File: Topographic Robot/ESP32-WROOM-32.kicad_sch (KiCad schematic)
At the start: 3 parts, among them U5 ESP32-WROOM-32

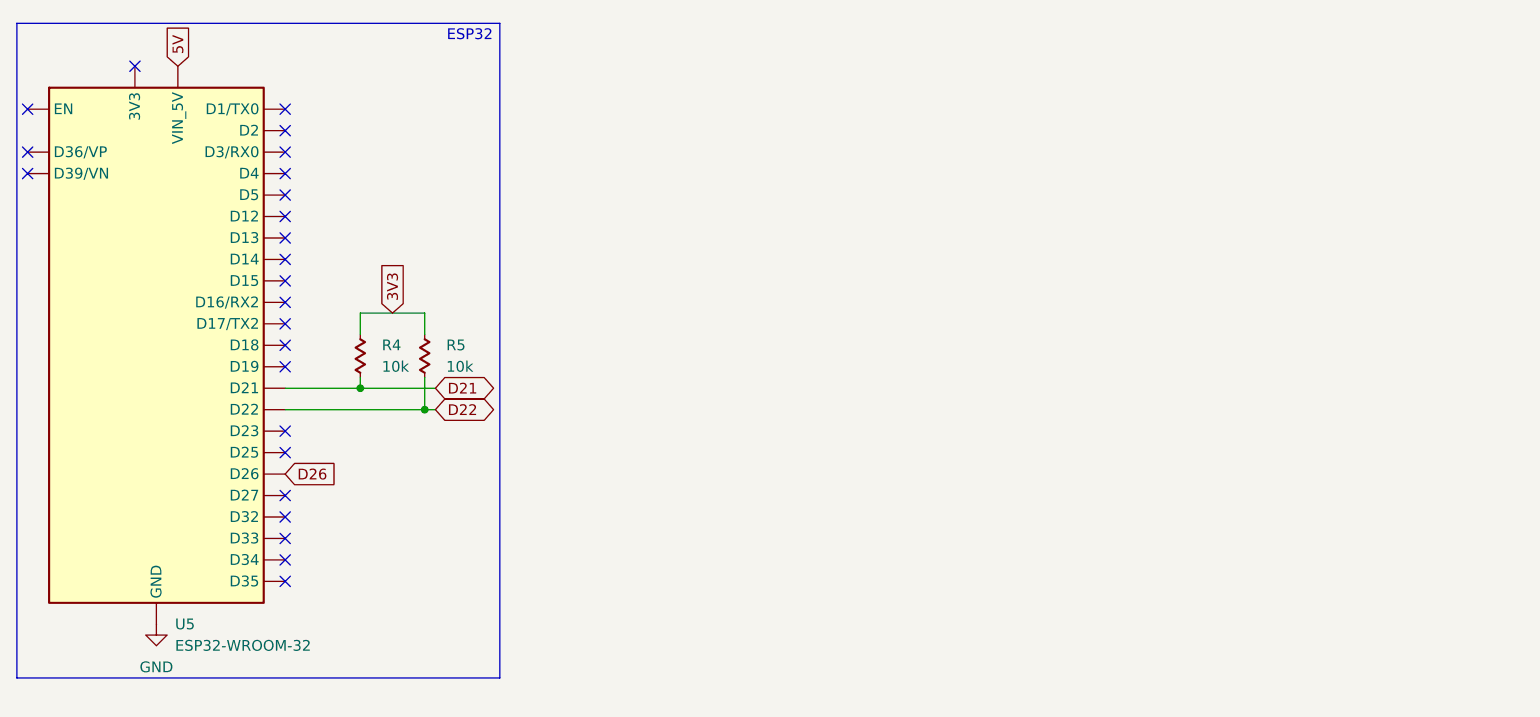
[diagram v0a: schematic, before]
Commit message: Movement + Sensors
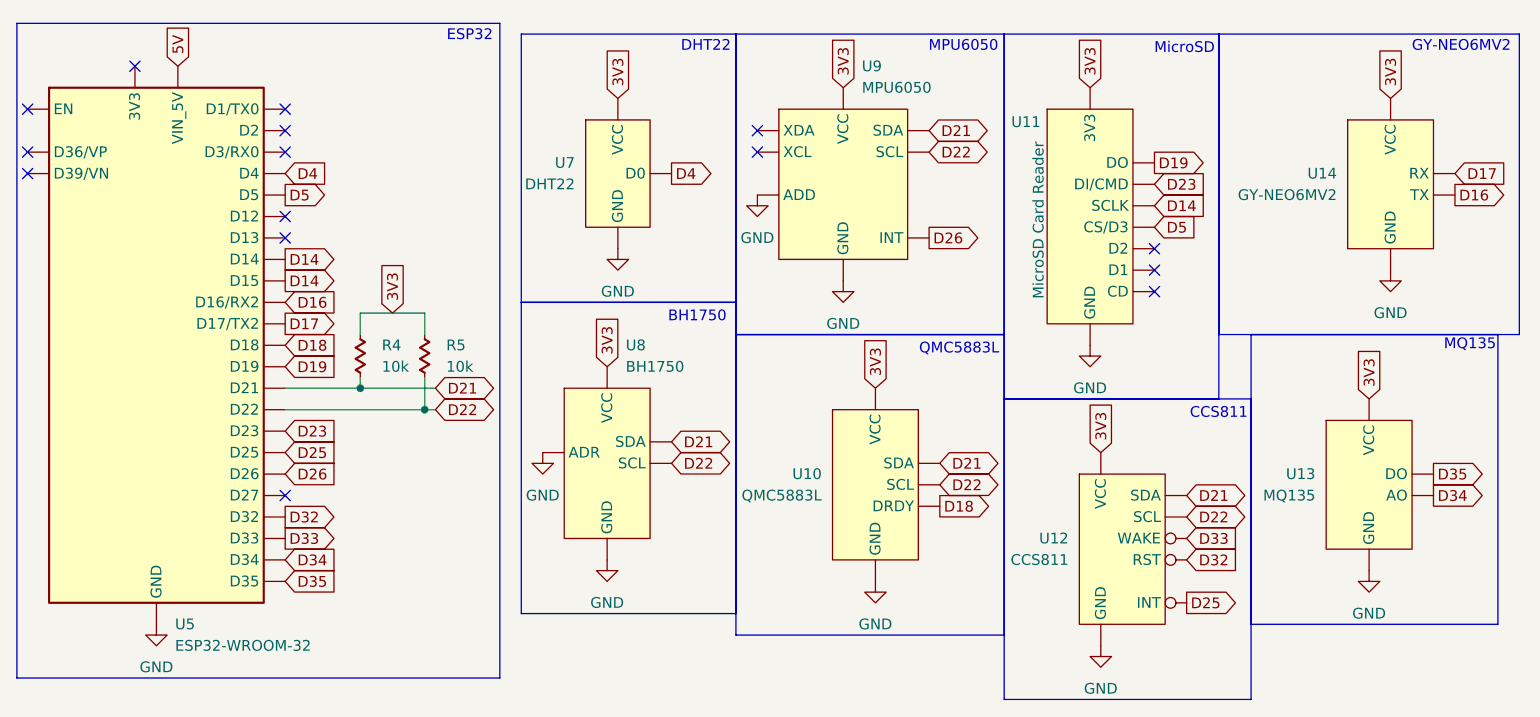
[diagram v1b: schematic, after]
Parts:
- added U10: QMC5883L, symbol Sensors:QMC5883L
- added U11: MicroSD Card Reader, symbol Sensors:MicroSD_Card_Reader
- added U12: CCS811, symbol Sensors:CCS811
- added U13: MQ135, symbol Sensors:MQ135
- added U14: GY-NEO6MV2, symbol Sensors:GY-NEO6MV2
- added U7: DHT22, symbol Sensors:DHT22
- added U8: BH1750, symbol Sensors:BH1750
- added U9: MPU6050, symbol Sensors:MPU6050
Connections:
- net 3V3: now also U10. (VCC), U11. (SCLK), U12. (WAKE), U13. (VCC), U14. (VCC), U7. (VCC), U8. (VCC), U9. (XDA)
- net D21: now also U10. (VCC), U12. (WAKE), U8. (VCC), U9. (XDA)
- net D22: now also U10. (VCC), U12. (WAKE), U8. (VCC), U9. (XDA)
- net D26: now also U9. (XDA)
- net GND: now also U10. (VCC), U11. (SCLK), U12. (WAKE), U13. (VCC), U14. (VCC), U7. (VCC), U8. (VCC), U9. (XDA)
- new net D14: U11. (SCLK), U5. (VIN_5V)
- new net D16: U14. (VCC), U5. (VIN_5V)
- new net D17: U14. (VCC), U5. (VIN_5V)
- new net D18: U10. (VCC), U5. (VIN_5V)
- new net D19: U11. (SCLK), U5. (VIN_5V)
- new net D23: U11. (SCLK), U5. (VIN_5V)
- new net D25: U12. (WAKE), U5. (VIN_5V)
- new net D32: U12. (WAKE), U5. (VIN_5V)
- new net D33: U12. (WAKE), U5. (VIN_5V)
- new net D34: U13. (VCC), U5. (VIN_5V)
- new net D35: U13. (VCC), U5. (VIN_5V)
- new net D4: U5. (VIN_5V), U7. (VCC)
- new net D5: U11. (SCLK), U5. (VIN_5V)
- no-connect marks 24 -> 15
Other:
- note added: "BH1750"
- note added: "CCS811"
- note added: "DHT22"
- note added: "GY-NEO6MV2"
- note added: "MPU6050"
- note added: "MQ135"
- note added: "MicroSD"
- note added: "QMC5883L"

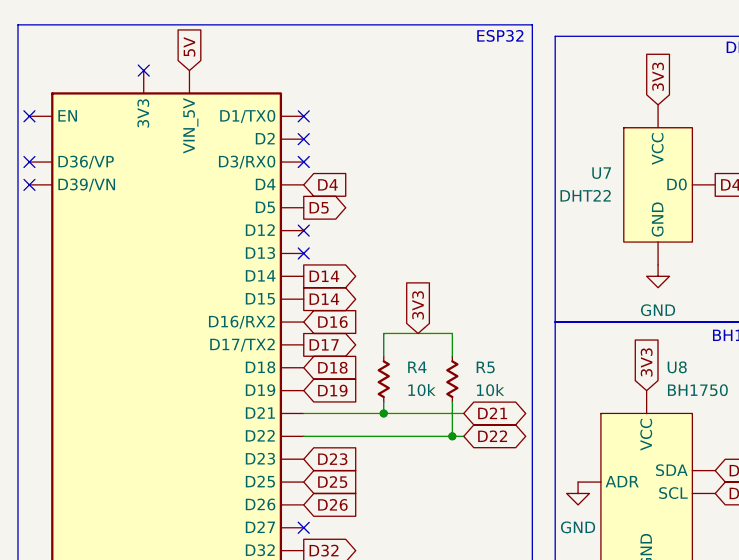
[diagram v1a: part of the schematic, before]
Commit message: THEY ARE QUAD TRISTATE BUFFERS TOOO SOOOOO I GOT 400 TRISTATE BUFFERS!!!!!
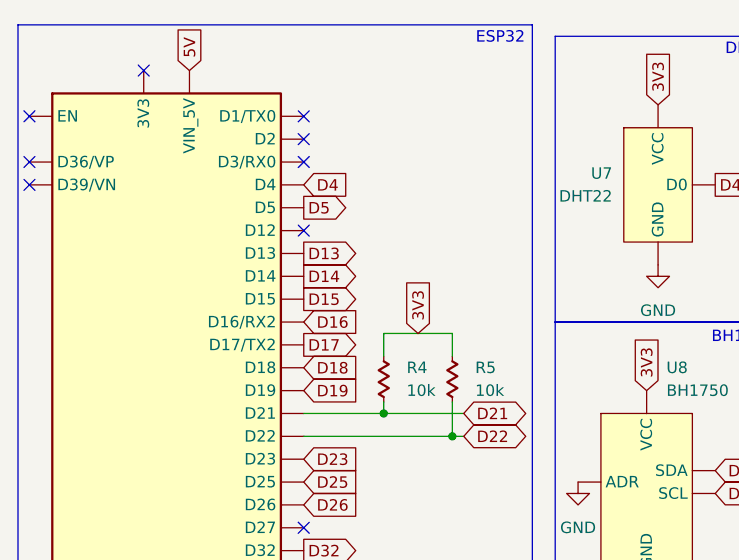
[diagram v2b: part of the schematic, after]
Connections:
- new net D13: U5. (VIN_5V)
- new net D15: U5. (VIN_5V)
- no-connect marks 15 -> 14
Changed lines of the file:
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@@
-	)
-	(no_connect
-		(at 44.45 38.1)
 	)
 	(no_connect
@@
 		)
 	)
-	(global_label "D14"
+	(global_label "D15"
 		(shape output)
 		(at 44.45 43.18 0)
@@
 			(effects
 				(font
+					(size 1.27 1.27)
+				)
+				(justify left)
+				(hide yes)
+			)
+		)
+	)
+	(global_label "D13"
+		(shape output)
+		(at 44.45 38.1 0)
+		(fields_autoplaced yes)
+		(effects
+			(font
+				(size 1.27 1.27)
+			)
+			(justify left)
+		)
+		(property "Intersheetrefs" "${INTERSHEET_REFS}"
+			(at 51.1242 38.1 0)
+			(effects
+				(font
